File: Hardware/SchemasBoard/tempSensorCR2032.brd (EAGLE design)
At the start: 36.1 x 22.6 mm, 11 parts, among them IC1 DS1820, T2 BC846

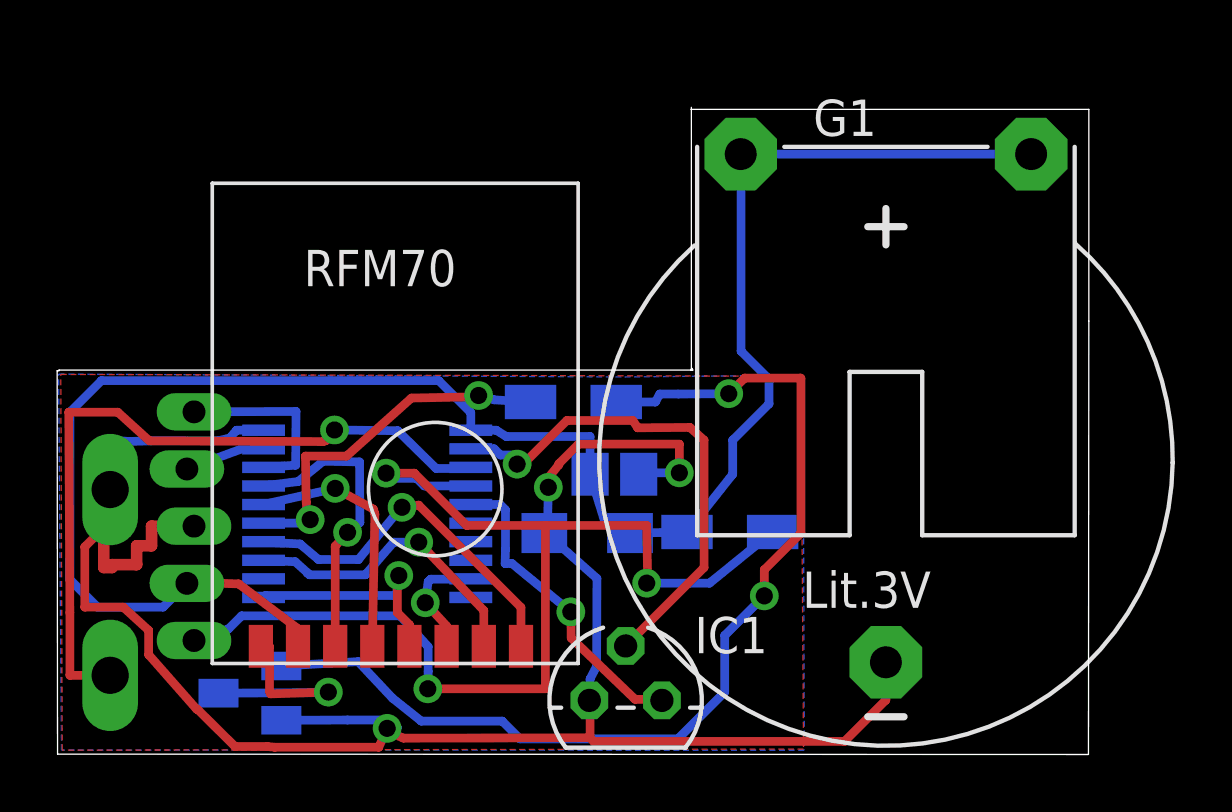
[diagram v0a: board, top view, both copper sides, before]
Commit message: hf
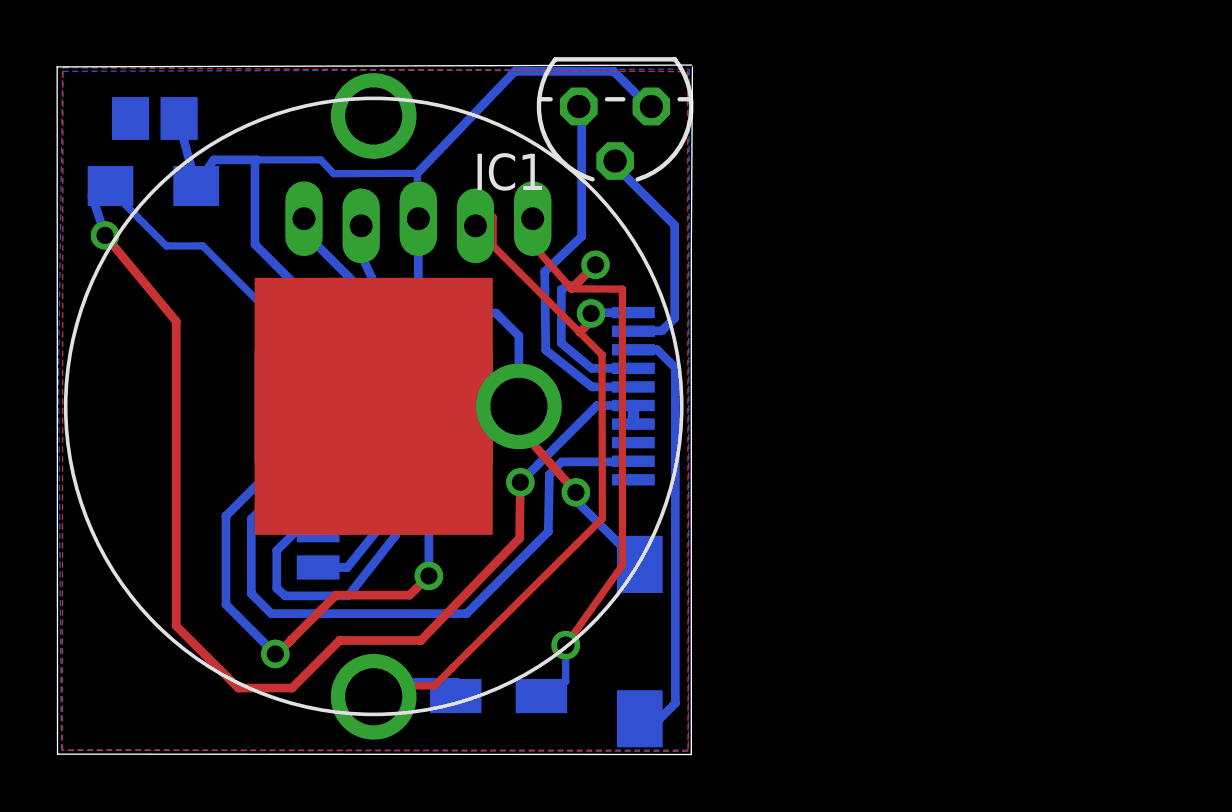
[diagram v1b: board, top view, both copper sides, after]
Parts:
- removed G1: CR2032H, battery:CR2032H
- removed R3: 1K, resistor:R1206W
- removed T2: BC846, transistor:SOT23
- added U$4: CR2032, rfm70:CR2032
- S1: value DTS-3 -> DTSM-3; device switch-tact:DTS-3 -> switch-tact:DTSM-3
- moved IC1 20.8 mm to (19.5, 22.7), turned to 180 degrees
- moved C1 20.3 mm to (3.40, 22.2)
- moved C2 19.4 mm to (3.35, 19.9), turned to 180 degrees
- moved S1 18.6 mm to (20.4, 3.94)
- moved U$3 13.3 mm to (12.6, 18.7), turned to 180 degrees
- moved U$1 12.7 mm to (-5.18, 15.5), flipped to the bottom, turned to 270 degrees
- moved R1 9.92 mm to (15.4, 2.03)
- moved U$2 7.02 mm to (16.5, 12.5)
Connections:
- removed net GND: C1.2, C2.-, G1.-, IC1.1, S1.1, T2.2, U$2.20, U$3.GND
- removed net N$13: T2.3, U$1.GND
- removed net N$14: R3.2, T2.1
- removed net N$15: R3.1, U$2.15
- new net N$4: C2.+, U$1.VDD, U$2.6, U$2.7
- new net N$5: R1.2, U$2.1, U$3.VDD, U$4.1
- new net VD: C1.2, C2.-, IC1.1, S1.1, U$1.GND, U$2.20, U$3.GND, U$4.3
- net VDD: no longer C2.+, G1.+, R1.2, U$1.VDD, U$2.1, U$3.VDD
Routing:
- net GND: track 73.1 -> 0.00 mm, vias 3 -> 0
- net VDD: track 66.4 -> 0.00 mm
- net N$4: track 0.00 -> 51.0 mm, vias 0 -> 2
- net VD: track 0.00 -> 45.6 mm, vias 0 -> 1
- net N$14: track 36.2 -> 0.00 mm, vias 2 -> 0
- net N$5: track 0.00 -> 29.5 mm, vias 0 -> 1
- net N$23: track 4.09 -> 22.3 mm, vias 1 -> 0
- net N$25: track 40.5 -> 27.5 mm, vias 3 -> 2
- net N$15: track 12.7 -> 0.00 mm, vias 2 -> 0
- net N$22: track 8.29 -> 19.6 mm, vias 1 -> 2
- net N$2: track 25.8 -> 14.9 mm, vias 1 -> 0
- net N$1: track 17.8 -> 7.99 mm, vias 1 -> 0
- net N$13: track 7.83 -> 0.00 mm, vias 1 -> 0
- net N$16: track 10.4 -> 3.97 mm, vias 1 -> 0
- net N$21: track 13.0 -> 8.11 mm, vias 1 -> 0
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- added copper zone on layer 1, net VD
- removed copper zone on layer 1, net GND
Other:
- board size 36.1 x 22.6 mm -> 22.2 x 24.1 mm
